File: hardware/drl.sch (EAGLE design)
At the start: 20 parts, among them IC1 TINY13-20SU, IC3 REG1117, Q1 IRF3205Z, Q2 IRF3205Z, T1 BC817-40, X1 CON1, X2 CON2

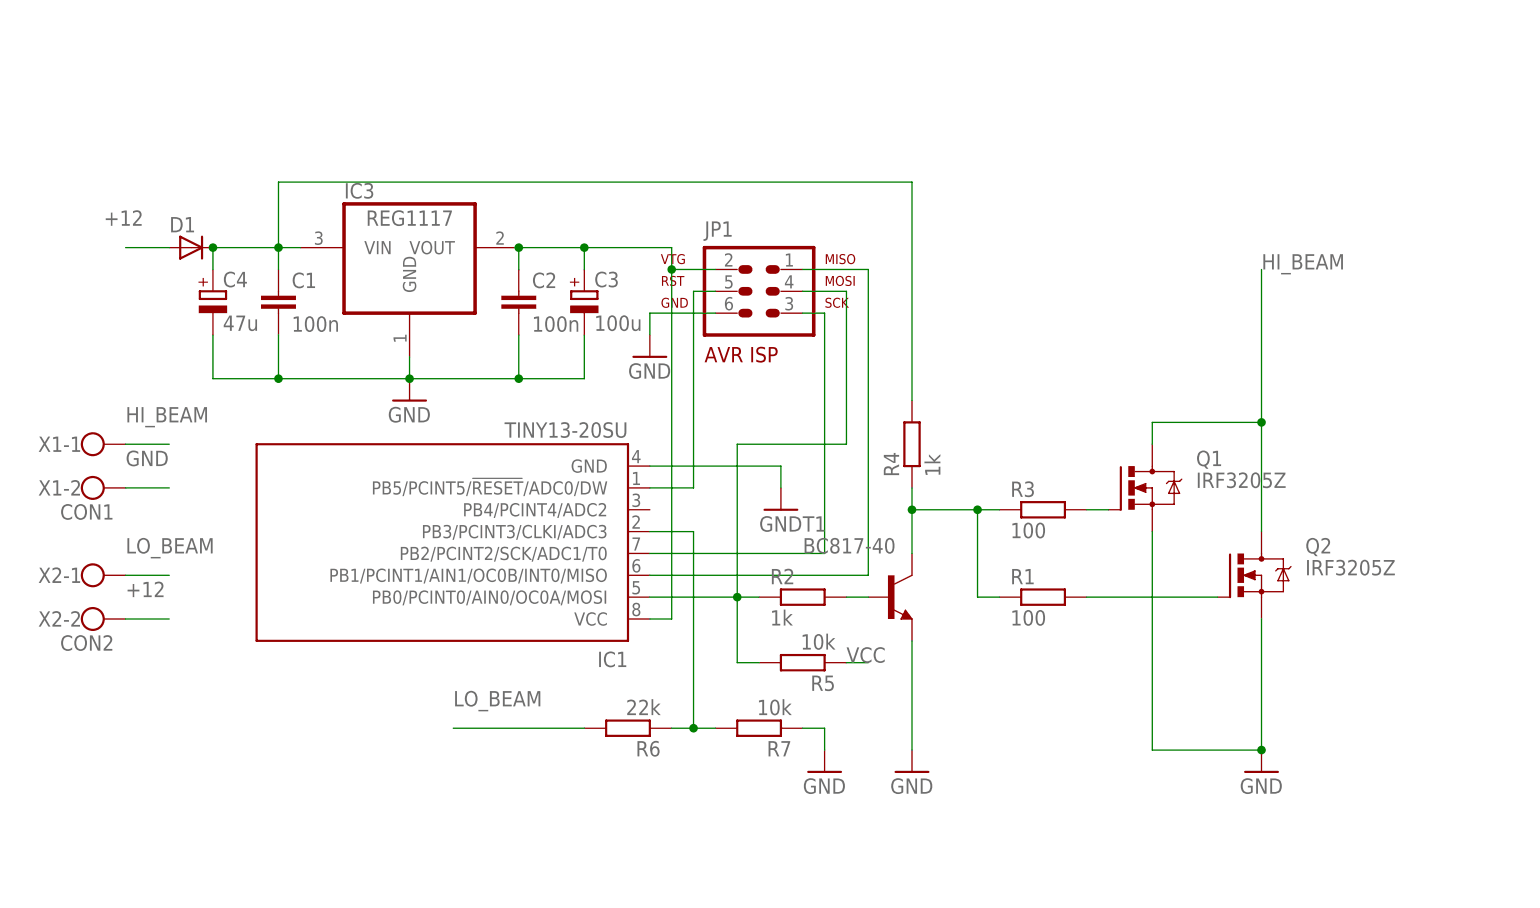
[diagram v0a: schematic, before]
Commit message: Second version of hardware (schematic and pcb)
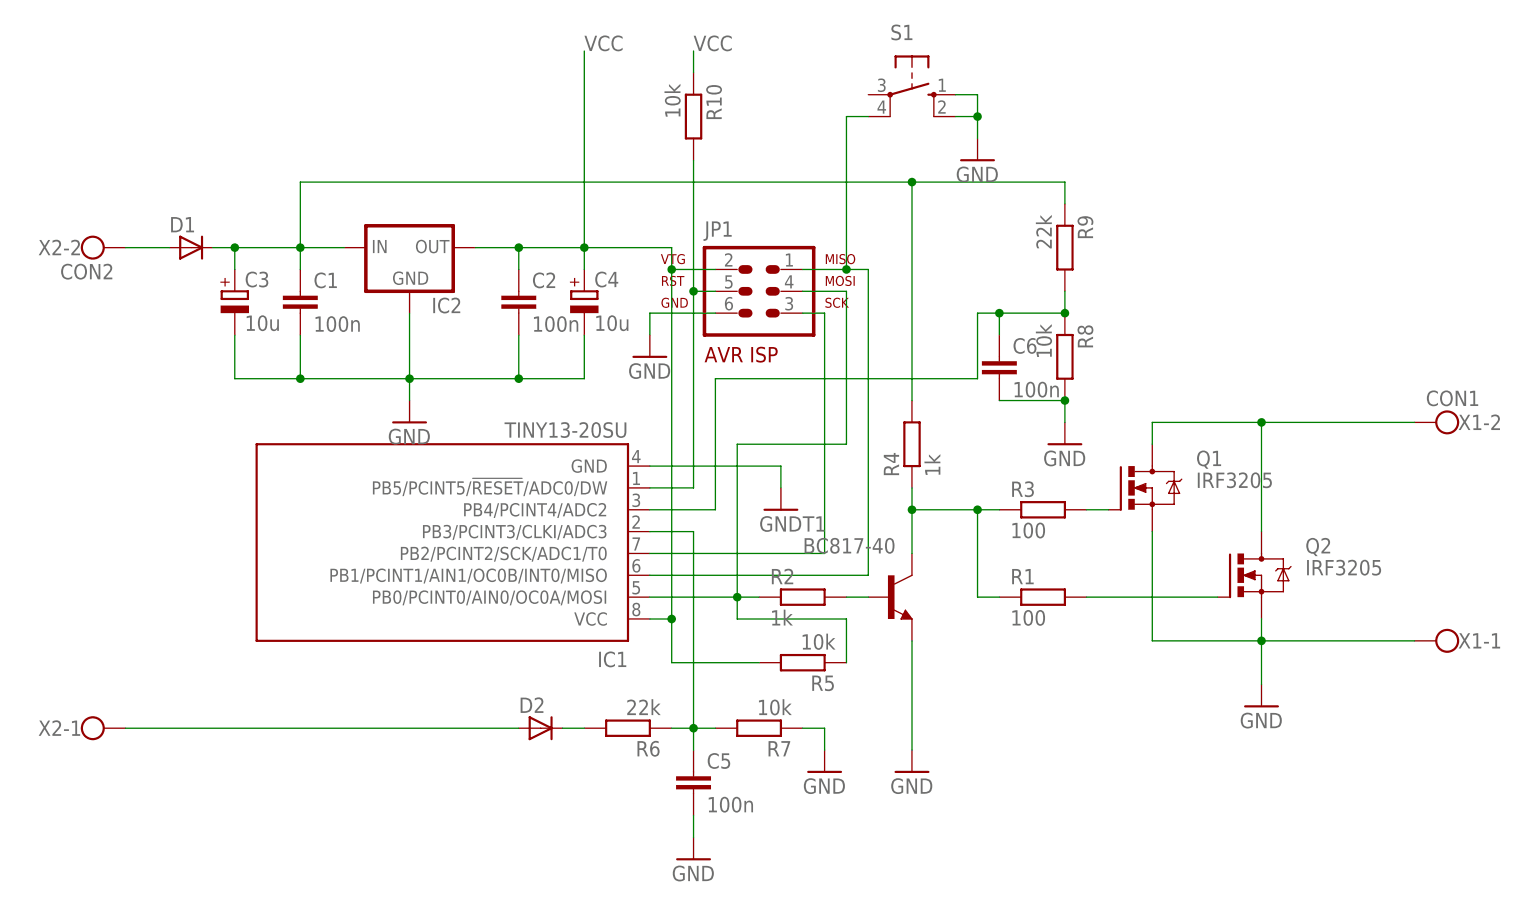
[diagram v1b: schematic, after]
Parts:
- removed IC3: REG1117, burr-brown:REG1117
- added C5, C6: 100n, resistor:C-EUC0805K
- added D2: (no value), semicon-smd-ipc:D-SOD-80
- added IC2: (no value), my_stuff:UA78L05SOIC
- added R10, R8: 10k, rcl:R-EU_R0805
- added R9: 22k, rcl:R-EU_R0805
- added S1: (no value), switch-omron:10-XX
- C3: value 100u -> 10u; device rcl:CPOL-EUE2,5-6E -> rcl:CPOL-EUSMCD
- C4: value 47u -> 10u; device rcl:CPOL-EUE2,5-6E -> rcl:CPOL-EUSMCD
- Q1, Q2: value IRF3205Z -> IRF3205; device my_stuff:IRF3205Z -> my_stuff:IRF3205
- R1: device rcl:R-EU_0204/7 -> rcl:R-EU_R0805
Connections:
- removed net LO_BEAM: R6.2, X2-1.KL
- removed net N$5: IC1.PB1/PCINT1/AIN1/OC0B/INT0/MISO, JP1.1
- new net N$11: IC1.PB0/PCINT0/AIN0/OC0A/MOSI, JP1.4, R2.1, R5.1
- new net N$12: IC1.PB1/PCINT1/AIN1/OC0B/INT0/MISO, JP1.1, S1.P1
- new net N$14: C6.1, IC1.PB4/PCINT4/ADC2, R8.1, R9.2
- new net N$2: D2.C, R6.2
- net GND: now also C5.2, C6.2, IC2.GND, R8.2, S1.S, S1.S1, X1-1.KL; no longer IC3.GND, X1-2.KL
- net HI_BEAM: now also X1-2.KL; no longer X1-1.KL
- net N$10: now also R10.2
- net N$7: now also D2.A, X2-1.KL; no longer IC1.PB0/PCINT0/AIN0/OC0A/MOSI, JP1.4, R2.1, R5.2
- net N$9: now also C5.1
- net VCC: now also C4.+, IC2.OUT, R10.1, R5.2; no longer C3.+, IC3.VOUT, R5.1
- net VCC12: now also C3.+, IC2.IN, R9.1; no longer C4.+, IC3.VIN
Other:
- moved on the sheet: C1, C3, C4, X1-1, X1-2, X2-1, X2-2

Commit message: Small editions in schematic and board design.
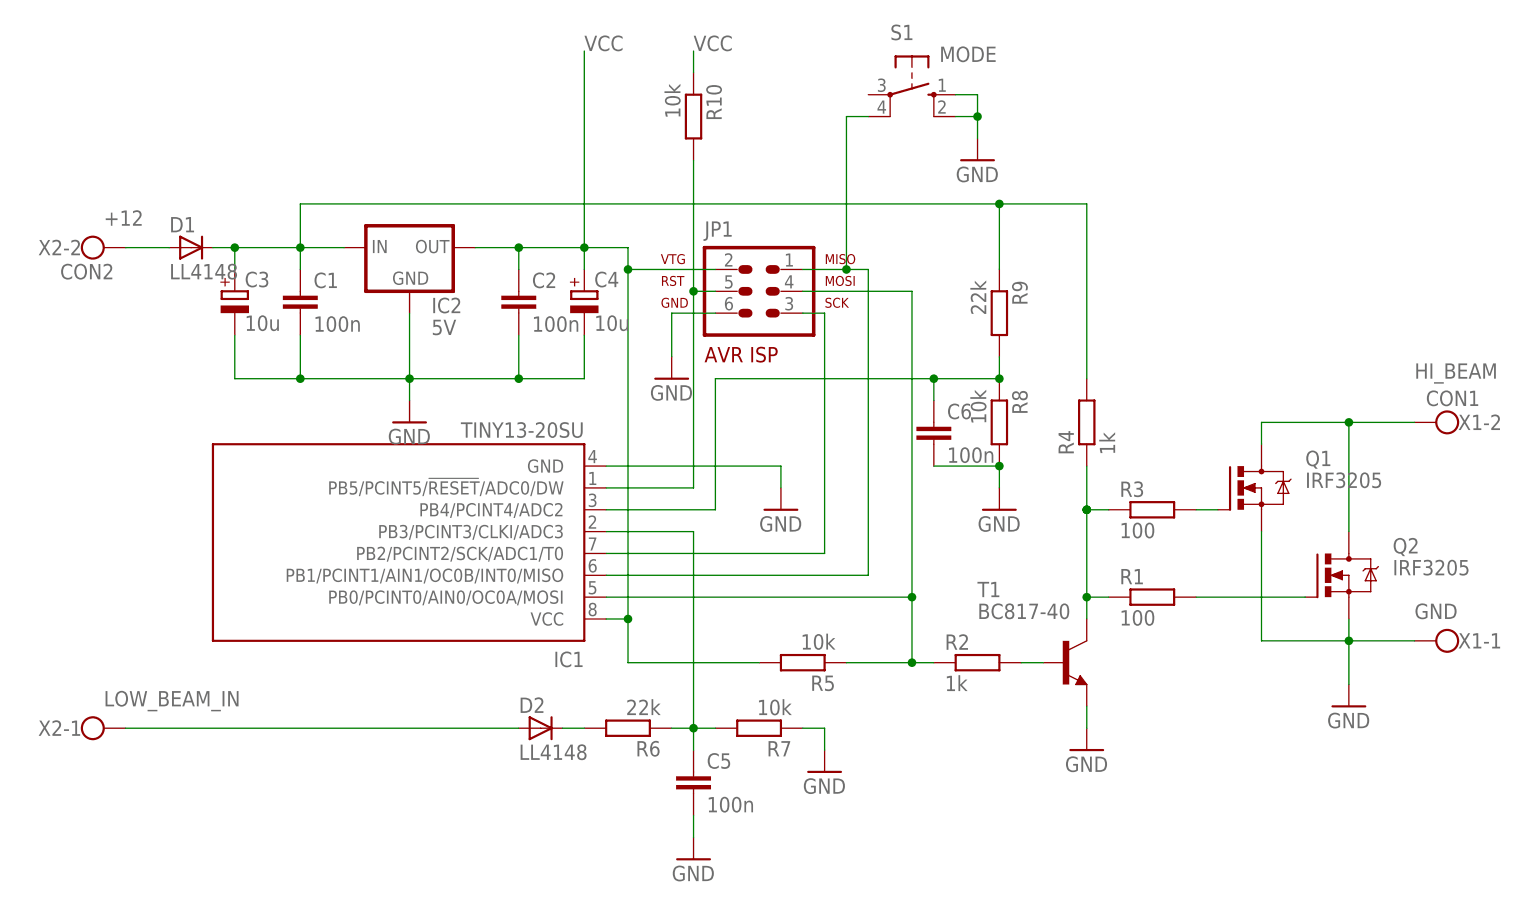
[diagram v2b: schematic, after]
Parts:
- D1, D2: value (none) -> LL4148
- IC2: value (none) -> 5V
- S1: value (none) -> MODE
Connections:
- net N$7 renamed LOW_BEAM_IN
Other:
- moved on the sheet: C6, IC1, Q1, Q2, R1, R2, R3, R4, R8, R9, T1
